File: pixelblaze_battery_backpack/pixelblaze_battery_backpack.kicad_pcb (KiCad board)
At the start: 4 copper layers, 76 x 42 mm, 60 parts, among them J1 Conn_01x01, J10 Conn_01x04, J11 Conn_01x04, J12 Conn_01x08, J13 Conn_01x04, J14 Conn_01x04, J15 Conn_01x04, J2 Conn_01x01, J3 Conn_01x01, J4 Conn_01x01, J5 USB_C_Receptacle_USB2.0_16P, J6 Conn_ARM_SWD_TagConnect_TC2030, J7 Conn_01x04, J8 Conn_QWIIC_Horizontal, J9 Conn_01x04, U1 HUSB238, U2 MSPM0C110xSRUK, U3 BQ25798, U4 LIS3DH, U5 TPS54560BDDA, U6 AP2112K-3.3

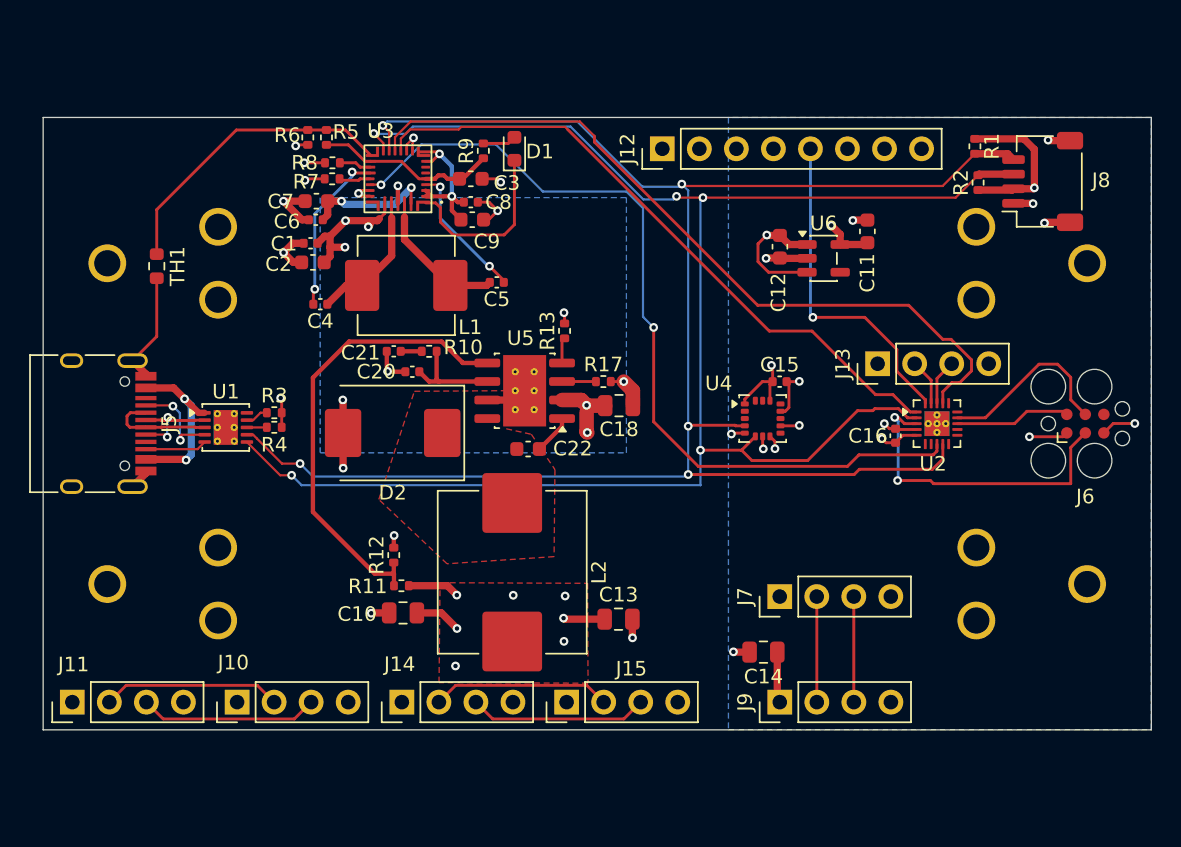
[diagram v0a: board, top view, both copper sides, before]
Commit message: Checkpoint, changing computers
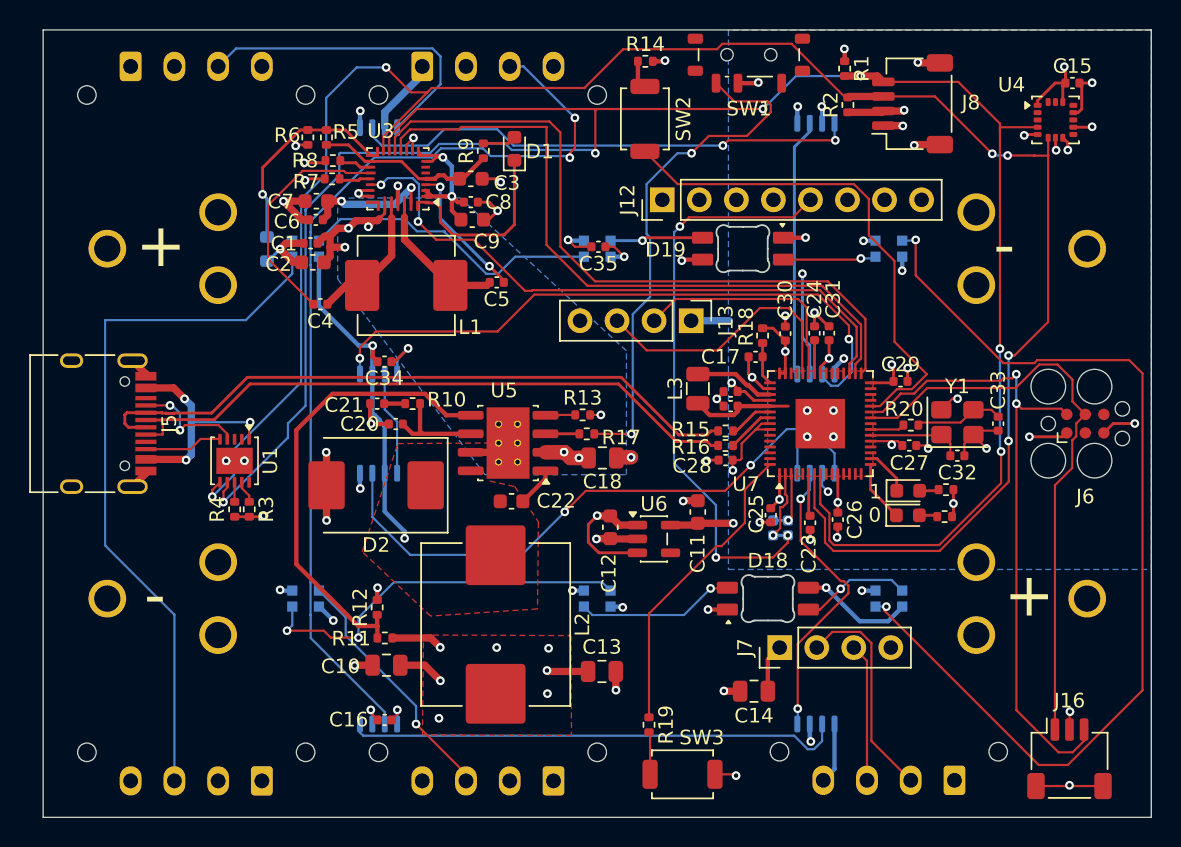
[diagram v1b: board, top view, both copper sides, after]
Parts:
- removed U2: MSPM0C110xSRUK, Package_DFN_QFN:Texas_RUK0020B_WQFN-20-1EP_3x3mm_P0.4mm_EP1.7x1.7mm_ThermalVias
- added C17: 4.7, Capacitor_SMD:C_0402_1005Metric, F.Cu at (98.9, 66.4)
- added C19: 4.7, Capacitor_SMD:C_0402_1005Metric, F.Cu at (97.2, 69.8)
- added C23: 0.1, Capacitor_SMD:C_0402_1005Metric, F.Cu at (102.6, 77.8)
- added C24: 0.1, Capacitor_SMD:C_0402_1005Metric, F.Cu at (102.9, 64.8)
- added C25: 0.1, Capacitor_SMD:C_0402_1005Metric, F.Cu at (99.9, 77.3)
- added C26: 0.1, Capacitor_SMD:C_0402_1005Metric, F.Cu at (104.5, 77.6)
- added C27: 0.1, Capacitor_SMD:C_0402_1005Metric, F.Cu at (109.4, 72.5)
- added C28: 0.1, Capacitor_SMD:C_0402_1005Metric, F.Cu at (96.8, 73.5)
- added C29: 0.1, Capacitor_SMD:C_0402_1005Metric, F.Cu at (108.8, 68.1)
- added C30: 0.1, Capacitor_SMD:C_0402_1005Metric, F.Cu at (100.9, 64.8)
- added C31: 0.1, Capacitor_SMD:C_0402_1005Metric, F.Cu at (103.9, 64.8)
- added C32: 15pF, Capacitor_SMD:C_0402_1005Metric, F.Cu at (112.7, 73.2)
- added C33: 15pF, Capacitor_SMD:C_0402_1005Metric, F.Cu at (115.5, 71.0)
- added C34: 4.7, Capacitor_SMD:C_0402_1005Metric, F.Cu at (73.4, 66.8)
- added C35: 4.7, Capacitor_SMD:C_0402_1005Metric, F.Cu at (88.1, 58.9)
- added C36: 4.7, Capacitor_SMD:C_0402_1005Metric, F.Cu at (97.2, 68.8)
- added D10: Xinglight_XL-4020RGBC-2812B, LED_SMD:LED_Xinglight_XL-4020RGBC-2812B_4x2mm_P0.85mm, B.Cu at (103.0, 50.7)
- added D11: Xinglight_XL-4020RGBC-2812B, LED_SMD:LED_Xinglight_XL-4020RGBC-2812B_4x2mm_P0.85mm, B.Cu at (103.0, 67.3)
- added D12: Xinglight_XL-4020RGBC-2812B, LED_SMD:LED_Xinglight_XL-4020RGBC-2812B_4x2mm_P0.85mm, B.Cu at (73.0, 67.3)
- added D13: Xinglight_XL-4020RGBC-2812B, LED_SMD:LED_Xinglight_XL-4020RGBC-2812B_4x2mm_P0.85mm, B.Cu at (73.0, 74.7)
- added D14: Xinglight_XL-4020RGBC-2812B, LED_SMD:LED_Xinglight_XL-4020RGBC-2812B_4x2mm_P0.85mm, B.Cu at (103.0, 74.7)
- added D15: Xinglight_XL-4020RGBC-2812B, LED_SMD:LED_Xinglight_XL-4020RGBC-2812B_4x2mm_P0.85mm, B.Cu at (103.0, 91.3)
- added D16: Xinglight_XL-4020RGBC-2812B, LED_SMD:LED_Xinglight_XL-4020RGBC-2812B_4x2mm_P0.85mm, B.Cu at (73.0, 91.3)
- added D17: LED_Small, LED_SMD:LED_0603_1608Metric, F.Cu at (109.3, 77.3)
- added D18: SK6812MINI-E, LED_SMD:LED_SK6812MINI-E_3.2x2.8mm_P1.5mm_ReverseMount, F.Cu at (99.7, 83.0)
- added D19: SK6812MINI-E, LED_SMD:LED_SK6812MINI-E_3.2x2.8mm_P1.5mm_ReverseMount, F.Cu at (98.0, 59.0)
- added D20: LED_Small, LED_SMD:LED_0603_1608Metric, F.Cu at (109.3, 75.6)
- added D3: WS2812B-2020, LED_SMD:LED_WS2812B-2020_PLCC4_2.0x2.0mm, B.Cu at (68.0, 83.0)
- added D4: Xinglight_XL-4020RGBC-2812B, LED_SMD:LED_Xinglight_XL-4020RGBC-2812B_4x2mm_P0.85mm, B.Cu at (73.0, 51.0)
- added D5: WS2812B-2020, LED_SMD:LED_WS2812B-2020_PLCC4_2.0x2.0mm, B.Cu at (88.0, 83.0)
- added D6: WS2812B-2020, LED_SMD:LED_WS2812B-2020_PLCC4_2.0x2.0mm, B.Cu at (108.0, 83.0)
- added D7: WS2812B-2020, LED_SMD:LED_WS2812B-2020_PLCC4_2.0x2.0mm, B.Cu at (108.0, 59.0)
- added D8: WS2812B-2020, LED_SMD:LED_WS2812B-2020_PLCC4_2.0x2.0mm, B.Cu at (88.0, 59.0)
- added D9: WS2812B-2020, LED_SMD:LED_WS2812B-2020_PLCC4_2.0x2.0mm, B.Cu at (68.0, 59.0)
- added J16: SM03B-SRSS-TB, Connector_JST:JST_SH_SM03B-SRSS-TB_1x03-1MP_P1.00mm_Horizontal, F.Cu at (120.4, 94.0)
- added L3: 3.3u, Inductor_SMD:L_0806_2016Metric, F.Cu at (94.9, 68.6)
- added R14: 1k, Resistor_SMD:R_0402_1005Metric, F.Cu at (91.3, 46.1)
- added R15: 27, Resistor_SMD:R_0402_1005Metric, F.Cu at (96.8, 71.5)
- added R16: 27, Resistor_SMD:R_0402_1005Metric, F.Cu at (96.8, 72.5)
- added R18: 27, Resistor_SMD:R_0402_1005Metric, F.Cu at (99.3, 65.0)
- added R19: 1k, Resistor_SMD:R_0402_1005Metric, F.Cu at (91.5, 91.7)
- added R20: 1k, Resistor_SMD:R_0402_1005Metric, F.Cu at (109.5, 71.1)
- added R21: RX_TX_Swap_SMD, SKEC_Footprints:RX_TX_SWAP_0402, B.Cu at (100.6, 78.2)
- added R22: 1k, Resistor_SMD:R_0402_1005Metric, F.Cu at (111.8, 77.4)
- added R23: 1k, Resistor_SMD:R_0402_1005Metric, F.Cu at (111.9, 75.5)
- added SW1: SW_SPDT, Button_Switch_SMD:SW_SPDT_Shouhan_MSK12C02, F.Cu at (98.4, 45.7)
- added SW2: SW_Push, Button_Switch_SMD:SW_SPST_TS-1088-xR020, F.Cu at (91.3, 50.1)
- added SW3: SW_Push, Button_Switch_SMD:SW_SPST_TS-1088-xR020, F.Cu at (93.8, 95.0)
- added U7: RP2354A, Package_DFN_QFN:QFN-60-1EP_7x7mm_P0.4mm_EP3.4x3.4mm, F.Cu at (103.3, 71.0)
- added Y1: 12MHz, Crystal:Crystal_SMD_3225-4Pin_3.2x2.5mm, F.Cu at (112.7, 70.9)
- C16: value 0.1 -> 4.7
- J10, J11, J14, J15, J9: footprint Connector_PinHeader_2.54mm:PinHeader_1x04_P2.54mm_Vertical -> Connector_Molex:Molex_Micro-Fit_3.0_43650-0415_1x04_P3.00mm_Vertical; moved to B.Cu
- TH1: moved to B.Cu
- U1: footprint Package_DFN_QFN:DFN-10-1EP_3x3mm_P0.5mm_EP1.65x2.38mm_ThermalVias -> Package_DFN_QFN:WDFN-10-1EP_3x3mm_P0.5mm_EP1.8x2.5mm
- moved J14 47.4 mm to (56.0, 46.5), turned to 0 degrees
- moved J15 44.7 mm to (76.0, 46.5), turned to 0 degrees
- moved C16 40.1 mm to (73.4, 91.3), turned to 0 degrees
- moved C15 28.7 mm to (120.6, 47.6)
- moved U4 28.7 mm to (119.4, 50.2)
- moved C11 22.5 mm to (94.9, 77.1)
- moved C12 22.5 mm to (88.9, 78.1)
- moved U6 22.5 mm to (91.9, 78.9)
- moved J10 22.4 mm to (85.0, 95.5), turned to 180 degrees
- moved J11 14.1 mm to (65.0, 95.5), turned to 180 degrees
- moved J13 13.1 mm to (94.4, 63.9), turned to -90 degrees
- moved J9 13.1 mm to (112.5, 95.5), turned to 180 degrees
- moved R1 10.4 mm to (105.0, 46.6)
- moved R2 10.4 mm to (105.2, 49.1)
- moved J8 10.4 mm to (109.6, 49.1)
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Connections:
- net /BATT+ renamed /Charger/BATT+
- net /CC1 renamed /USB_Input/CC1
- net /CC2 renamed /USB_Input/CC2
- net /PMID renamed /Charger/PMID
- net /REGN renamed /Charger/REGN
- net /STAT renamed /Charger/STAT
- C16 pad 1: +3V3 -> +5V
- J10 pad 2: /Pixel_CLK2 -> /Battery LEDs/Pixel_CLK2
- J10 pad 3: /Pixel_DAT2 -> /Battery LEDs/Pixel_DAT2
- J11 pad 2: /Pixel_CLK2 -> unconnected-(J11-Pin_2-Pad2)
- J11 pad 3: /Pixel_DAT2 -> Net-(D9-DOUT)
- J13 pad 2: /MSP_A1 -> /MCU/ADC0
- J13 pad 3: /MSP_A2 -> /MCU/ADC1
- J14 pad 2: /Pixel_CLK3 -> /Battery LEDs/Pixel_CLK3
- J14 pad 3: /Pixel_DAT3 -> /Battery LEDs/Pixel_DAT3
- J15 pad 2: /Pixel_CLK3 -> unconnected-(J15-Pin_2-Pad2)
- J15 pad 3: /Pixel_DAT3 -> Net-(D16-DO)
- J6 pad 2: /SWDIO -> /MCU/SWDIO
- J6 pad 3: /~{NRST} -> /MCU/~{NRST}
- J6 pad 4: /SWCLK -> /MCU/SWCLK
- R17 pad 2: GND -> Net-(SW1-C)
- U1 pad 2: /D+ -> unconnected-(U1-D+-Pad2)
- U1 pad 3: /D- -> unconnected-(U1-D--Pad3)
- U3 pad 12: /~{QON} -> /~{BQ_QON}
- U3 pad 13: /~{CE} -> /~{BQ_CE}
- U3 pad 21: /~{INT} -> /~{BQ_INT}
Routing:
- net Net-(D6-DOUT): track 0.00 -> 68.9 mm, vias 0 -> 2
- net Net-(D16-DO): track 0.00 -> 65.6 mm, vias 0 -> 2
- net /~{INT}: track 58.2 -> 0.00 mm, vias 2 -> 0
- net +5V: track 21.9 -> 78.4 mm, vias 8 -> 21
- net GND: track 66.1 -> 119.0 mm, vias 29 -> 64
- net /~{CE}: track 52.1 -> 0.00 mm
- net Net-(D9-DOUT): track 0.00 -> 48.9 mm
- net /~{BQ_CE}: track 0.00 -> 47.7 mm
- net /~{BQ_QON}: track 0.00 -> 46.6 mm
- net /MCU/SWDIO: track 0.00 -> 44.8 mm, vias 0 -> 2
- net /~{QON}: track 44.7 -> 0.00 mm
- net Net-(D11-DO): track 0.00 -> 43.9 mm, vias 0 -> 2
- net /~{BQ_INT}: track 0.00 -> 42.8 mm, vias 0 -> 2
- net Net-(D13-DO): track 0.00 -> 41.4 mm, vias 0 -> 2
- net /MCU/SWCLK: track 0.00 -> 41.0 mm
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- added copper zone on F.Cu, net +1V1
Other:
- board size 76 x 42 mm -> 76 x 54 mm
- board text added: "${TITLE} V${REVISION}"
- board text added: "+"
- board text added: "-"
- board text added: "0"
- board text added: "1"
- board text added: "LED IN"
- board text added: "LED OUT"
- board text added: "SKEC"
